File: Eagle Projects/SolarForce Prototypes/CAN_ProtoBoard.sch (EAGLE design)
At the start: 18 parts, among them U1 MCP2551

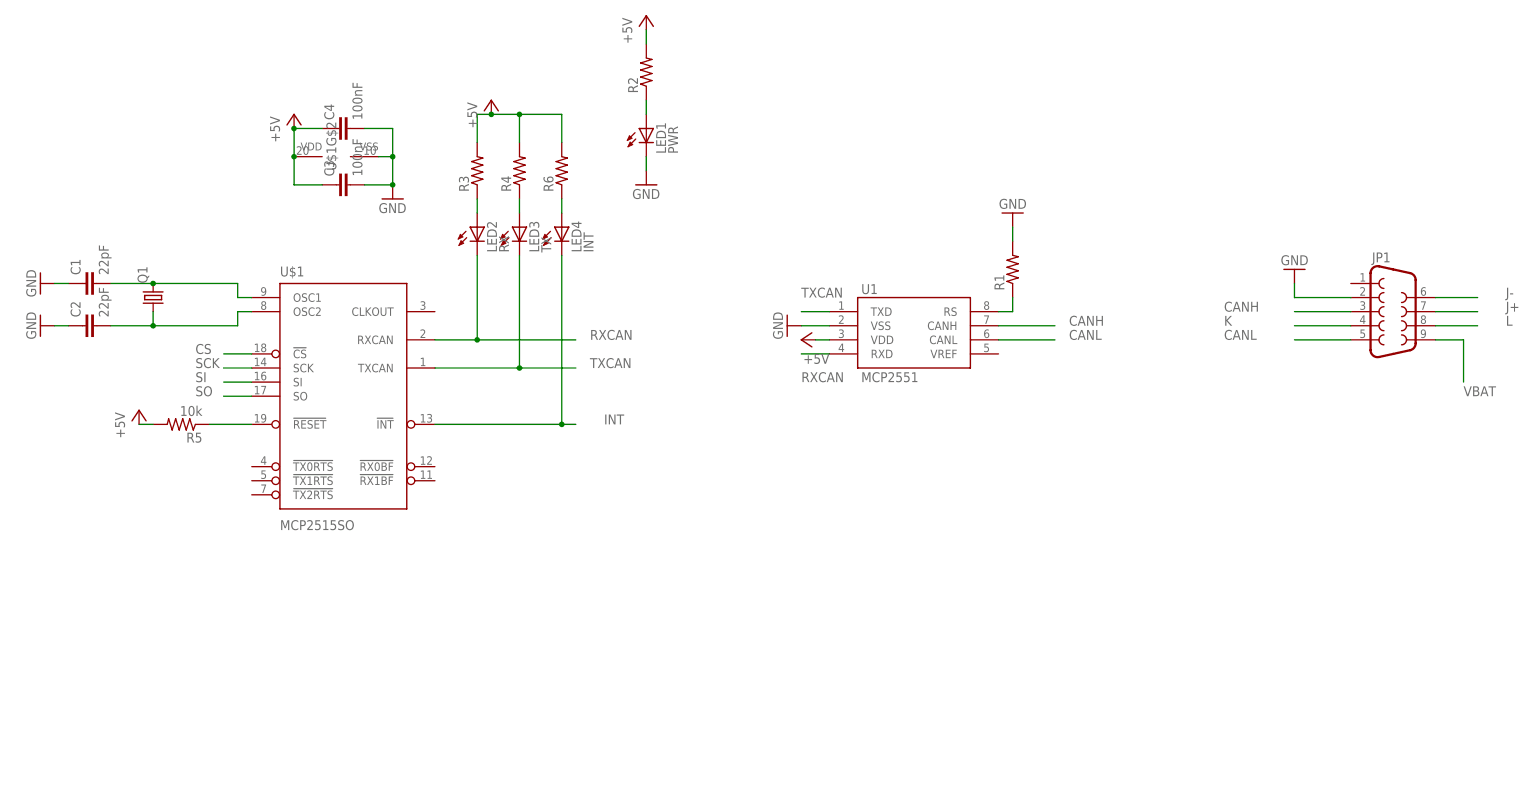
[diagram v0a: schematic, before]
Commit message: CAN ProtoPCB V1 Ready..
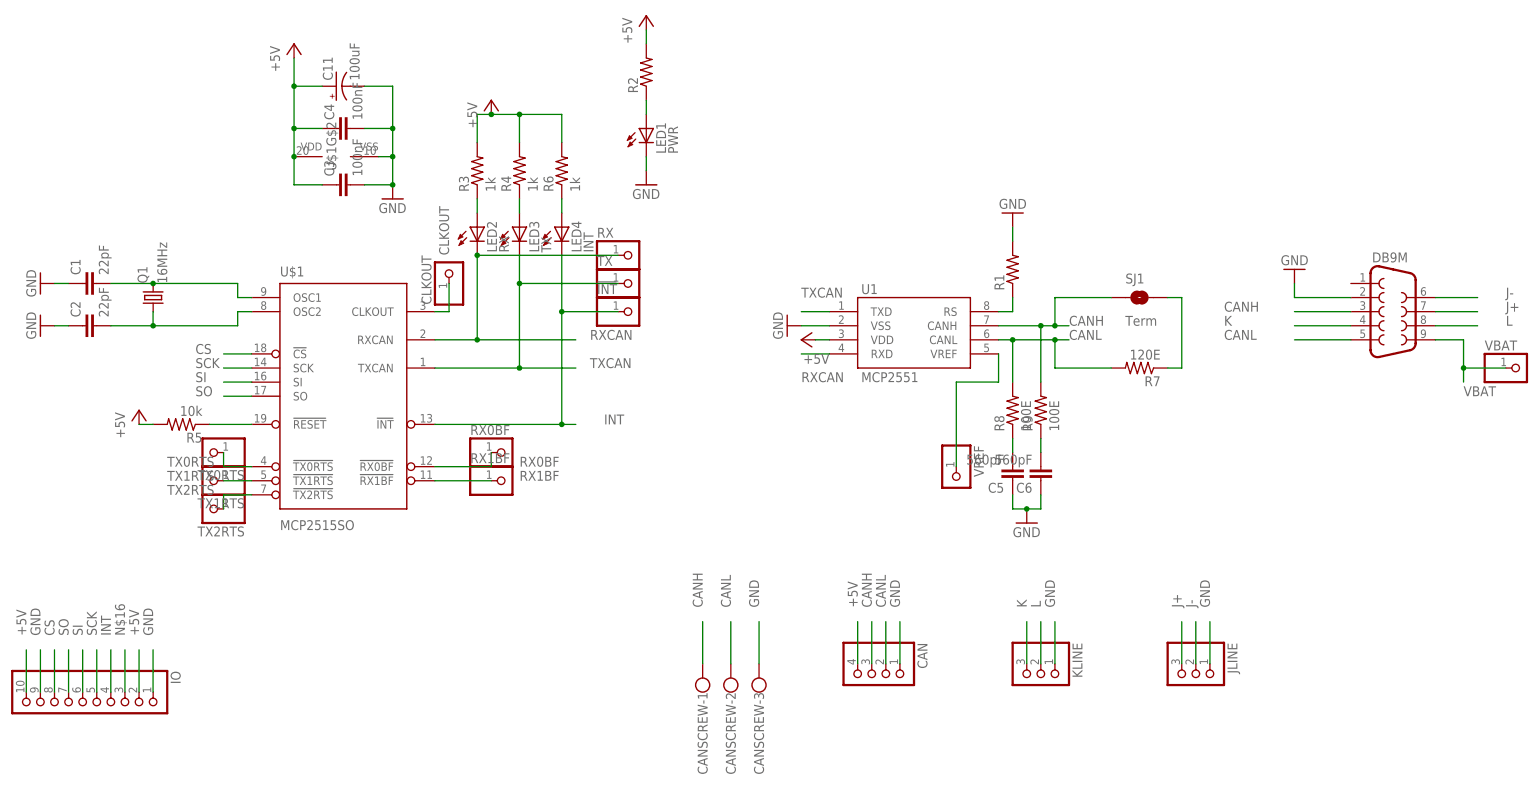
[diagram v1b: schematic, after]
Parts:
- added !INT, CLKOUT, RX, RX0BF, RX1BF, TX, TX0RTS, TX1RTS, TX2RTS, VBAT, VREF: (no value), pinhead:PINHD-1X1
- added C11: 100uF, resistor:CPOL-USD
- added C5, C6: 560pF, resistor:C-EUC0805K
- added CAN: (no value), pinhead:PINHD-1X4
- added CANSCREW: (no value), con-wago-500:W237-103
- added IO: (no value), pinhead:PINHD-1X10
- added JLINE, KLINE: (no value), pinhead:PINHD-1X3
- added R7: 120E, resistor:R-US_R0805
- added R8, R9: 100E, resistor:R-US_R0805
- added SJ1: Term, SparkFun-Retired:SOLDERJUMPERTRACE
- Q1: value (none) -> 16MHz
- R3, R4, R6: value (none) -> 1k
- renumbered JP1 to DB9M
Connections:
- new net CLKOUT: CLKOUT.1, U$1G$1.CLKOUT
- new net N$10: U1.VREF, VREF.1
- new net N$11: C5.2, R8.1
- new net N$12: C6.2, R9.1
- new net N$16: IO.3
- new net N$9: R7.1, SJ1.2
- new net RX0BF: RX0BF.1, U$1G$1.!RX0BF
- new net RX1BF: RX1BF.1, U$1G$1.!RX1BF
- new net TX0RTS: TX0RTS.1, U$1G$1.!TX0RTS
- new net TX1RTS: TX1RTS.1, U$1G$1.!TX1RTS
- new net TX2RTS: TX2RTS.1, U$1G$1.!TX2RTS
- net +5V: now also C11.+, CAN.4, IO.10, IO.2
- net CANH: now also CAN.3, CANSCREW-1.KL, R9.2, SJ1.1
- net CANL: now also CAN.2, CANSCREW-2.KL, R7.2, R8.2
- net CS: now also IO.8
- net GND: now also C11.-, C5.1, C6.1, CAN.1, CANSCREW-3.KL, IO.1, IO.9, JLINE.1, KLINE.1
- net INT: now also !INT.1, IO.4
- net J+: now also JLINE.3
- net J-: now also JLINE.2
- net K: now also KLINE.3
- net L: now also KLINE.2
- net RXCAN: now also RX.1
- net SCK: now also IO.5
- net SI: now also IO.6
- net SO: now also IO.7
- net TXCAN: now also TX.1
- net VBAT: now also VBAT.1
